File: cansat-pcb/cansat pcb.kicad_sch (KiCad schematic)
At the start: 3 parts, among them J1 Conn_01x02_Pin, SW1 SW_DPDT_x2

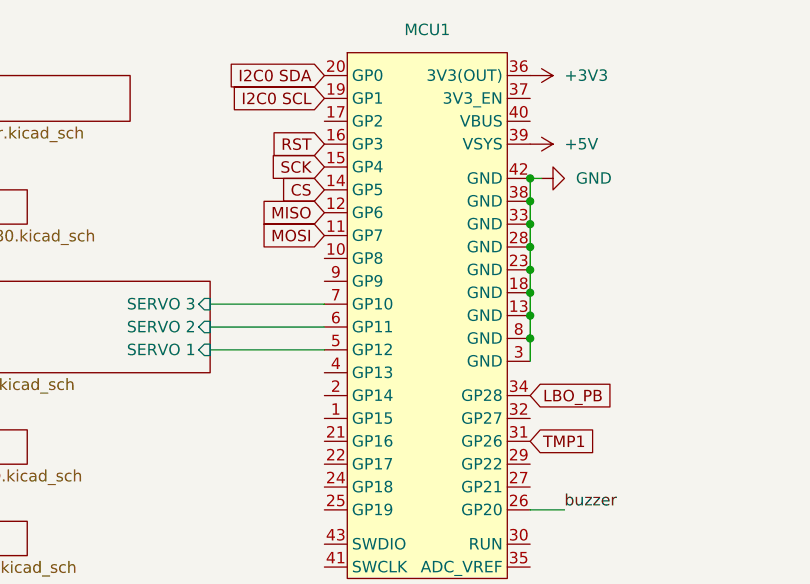
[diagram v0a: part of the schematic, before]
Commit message: pcb V2
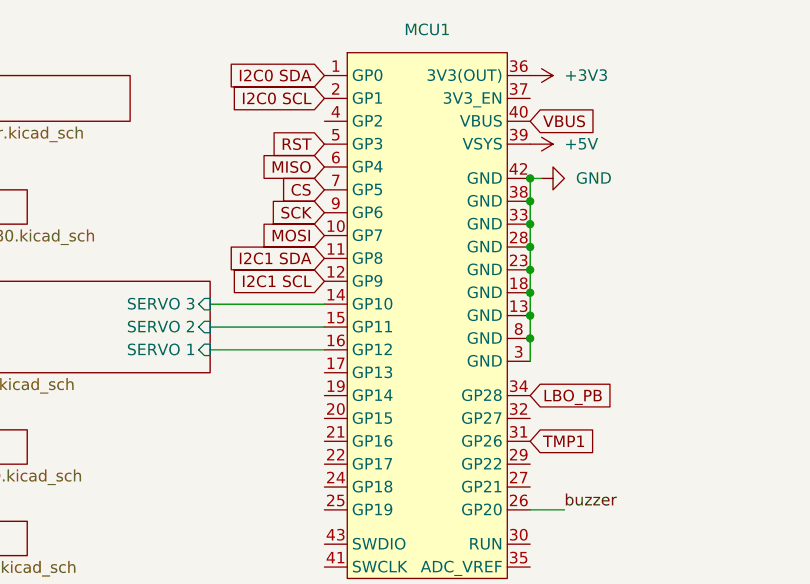
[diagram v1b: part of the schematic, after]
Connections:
- net CS: now also MCU1.7 (GP5); no longer MCU1.14 (GP5)
- net I2C0 SCL: now also MCU1.2 (GP1); no longer MCU1.19 (GP1)
- net I2C0 SDA: now also MCU1.1 (GP0); no longer MCU1.20 (GP0)
- net MISO: now also MCU1.6 (GP4); no longer MCU1.12 (GP6)
- net MOSI: now also MCU1.10 (GP7); no longer MCU1.11 (GP7)
- net RST: now also MCU1.5 (GP3); no longer MCU1.16 (GP3)
- net SCK: now also MCU1.9 (GP6); no longer MCU1.15 (GP4)
- net SERVO/SERVO 1: now also MCU1.16 (GP12); no longer MCU1.5 (GP12)
- net SERVO/SERVO 2: now also MCU1.15 (GP11); no longer MCU1.6 (GP11)
- net SERVO/SERVO 3: now also MCU1.14 (GP10); no longer MCU1.7 (GP10)
- net VBUS: now reaches MCU1.40 (VBUS)
- new net I2C1 SCL: MCU1.12 (GP9)
- new net I2C1 SDA: MCU1.11 (GP8)
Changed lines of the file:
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@@
     )
   )
-  (global_label "MISO" (shape input) (at 95.25 55.88 180) (fields_autoplaced)
+  (global_label "I2C1 SDA" (shape input) (at 95.25 60.96 180) (fields_autoplaced)
     (effects (font (size 1.27 1.27)) (justify right))
-    (property "Intersheetrefs" "${INTERSHEET_REFS}" (at 87.6686 55.88 0)
+    (property "Intersheetrefs" "${INTERSHEET_REFS}" (at 84.0895 60.96 0)
+      (effects (font (size 1.27 1.27)) (justify right) hide)
+    )
+  )
+  (global_label "I2C1 SCL" (shape input) (at 95.25 63.5 180) (fields_autoplaced)
+    (effects (font (size 1.27 1.27)) (justify right))
+    (property "Intersheetrefs" "${INTERSHEET_REFS}" (at 84.15 63.5 0)
+      (effects (font (size 1.27 1.27)) (justify right) hide)
+    )
+  )
+  (global_label "MISO" (shape input) (at 95.25 50.8 180) (fields_autoplaced)
+    (effects (font (size 1.27 1.27)) (justify right))
+    (property "Intersheetrefs" "${INTERSHEET_REFS}" (at 87.6686 50.8 0)
       (effects (font (size 1.27 1.27)) (justify right) hide)
     )
@@
     )
   )
+  (global_label "VBUS" (shape input) (at 118.11 45.72 0) (fields_autoplaced)
+    (effects (font (size 1.27 1.27)) (justify left))
+    (property "Intersheetrefs" "${INTERSHEET_REFS}" (at 125.3396 45.72 0)
+      (effects (font (size 1.27 1.27)) (justify left) hide)
+    )
+  )
   (global_label "MOSI" (shape input) (at 95.25 58.42 180) (fields_autoplaced)
     (effects (font (size 1.27 1.27)) (justify right))
@@
     )
   )
-  (global_label "SCK" (shape input) (at 95.25 50.8 180) (fields_autoplaced)
+  (global_label "SCK" (shape input) (at 95.25 55.88 180) (fields_autoplaced)
     (effects (font (size 1.27 1.27)) (justify right))
-    (property "Intersheetrefs" "${INTERSHEET_REFS}" (at 88.5153 50.8 0)
+    (property "Intersheetrefs" "${INTERSHEET_REFS}" (at 88.5153 55.88 0)
       (effects (font (size 1.27 1.27)) (justify right) hide)
     )
